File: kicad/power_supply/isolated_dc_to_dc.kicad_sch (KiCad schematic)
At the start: 23 parts, among them U1001 LM25184NGUR, U1002 750313445

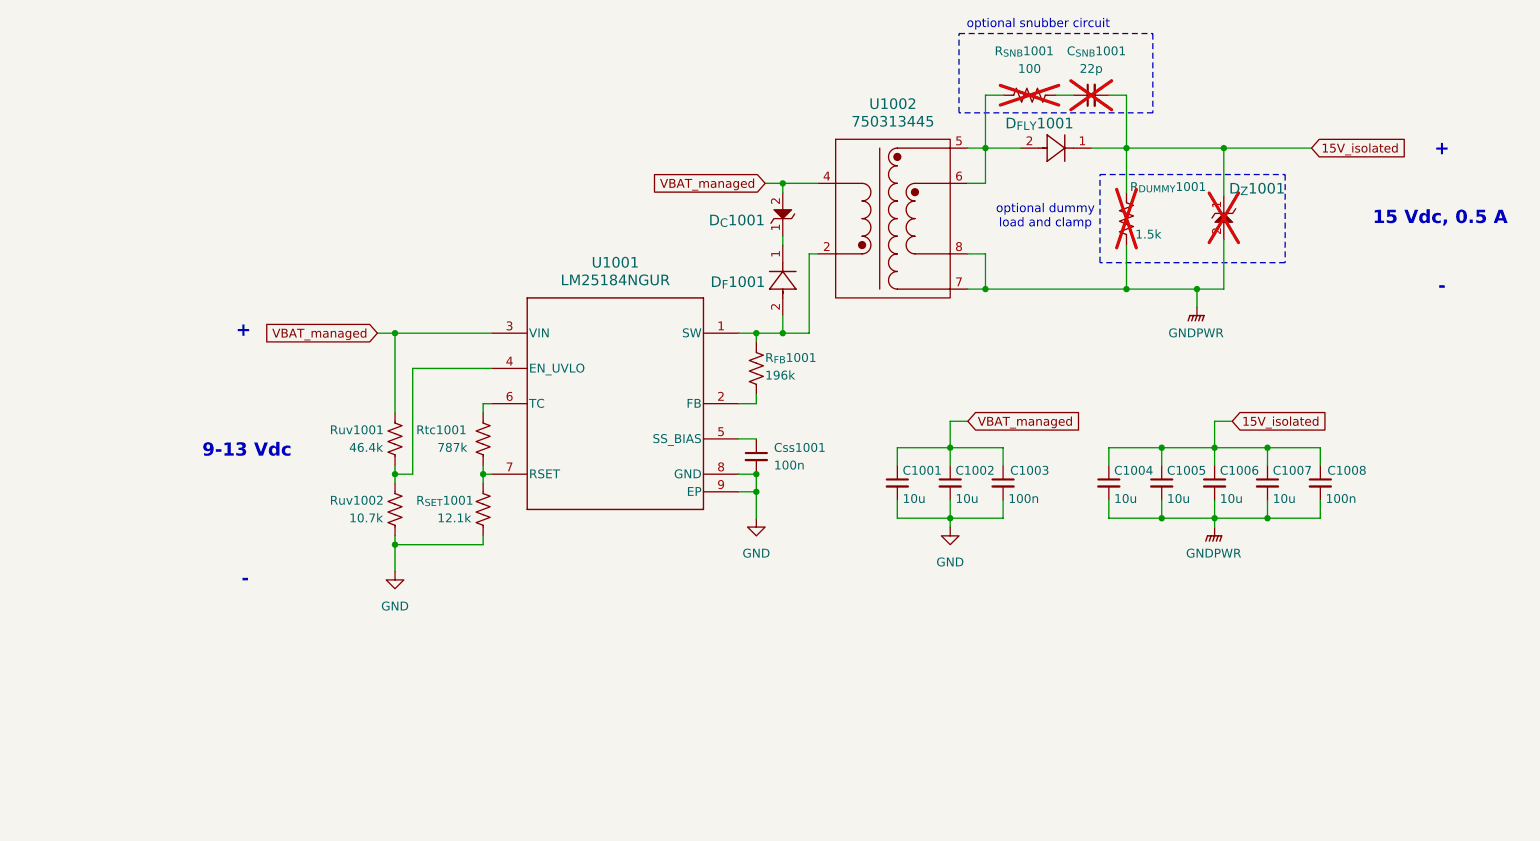
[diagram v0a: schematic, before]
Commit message: psu
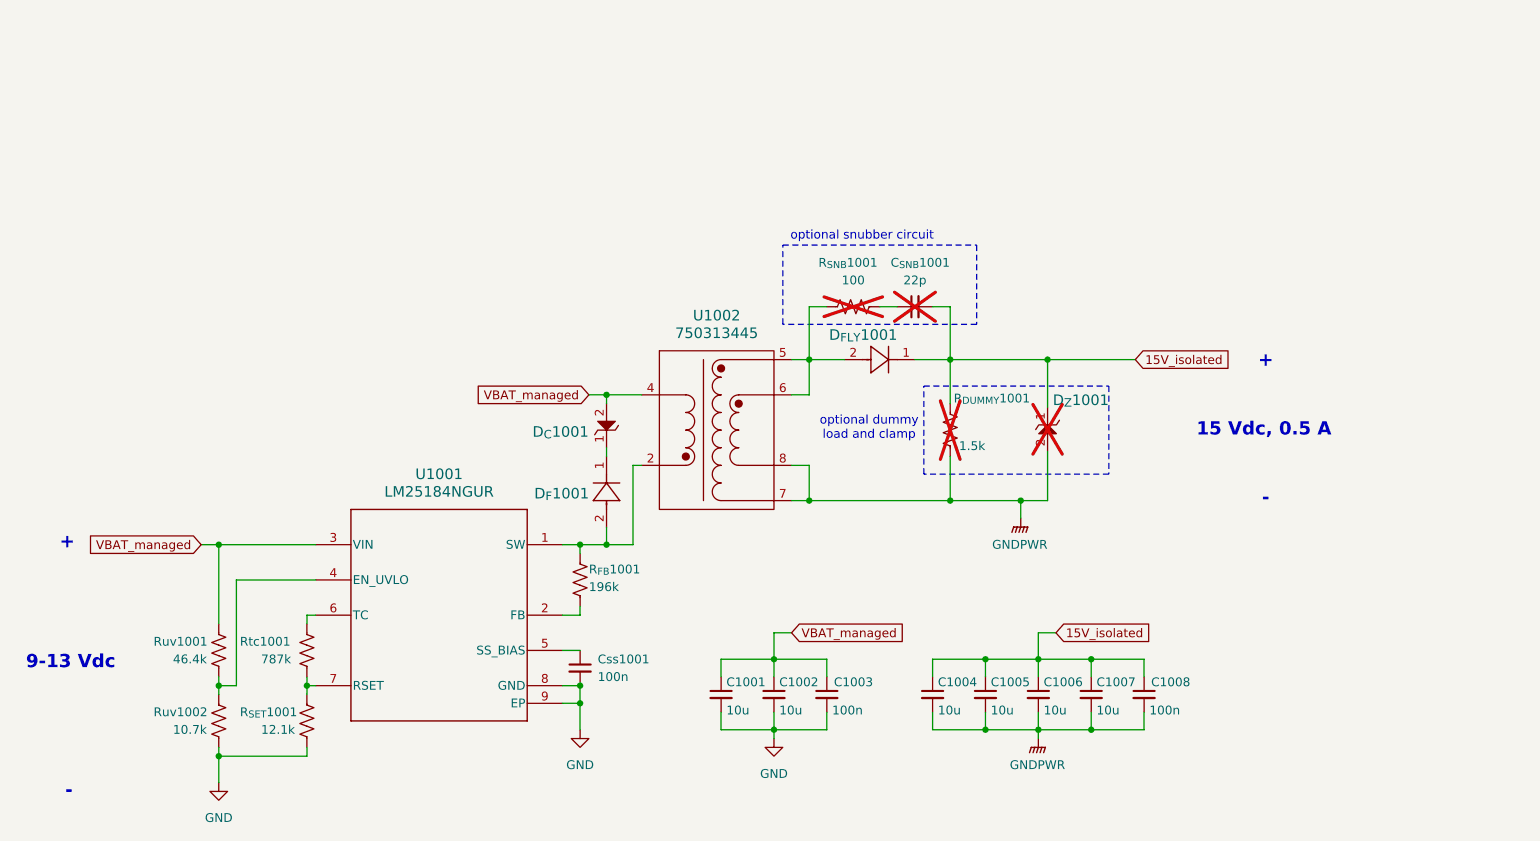
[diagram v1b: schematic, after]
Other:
- moved on the sheet: C1001, C1002, C1003, C1004, C1005, C1006, C1007, C1008, C_{SNB}1001, Css1001, D_{C}1001, D_{FLY}1001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
